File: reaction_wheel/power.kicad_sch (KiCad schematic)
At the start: 20 parts, among them U10 TPS62902RPJR, U11 TPS61379QWRTERQ1

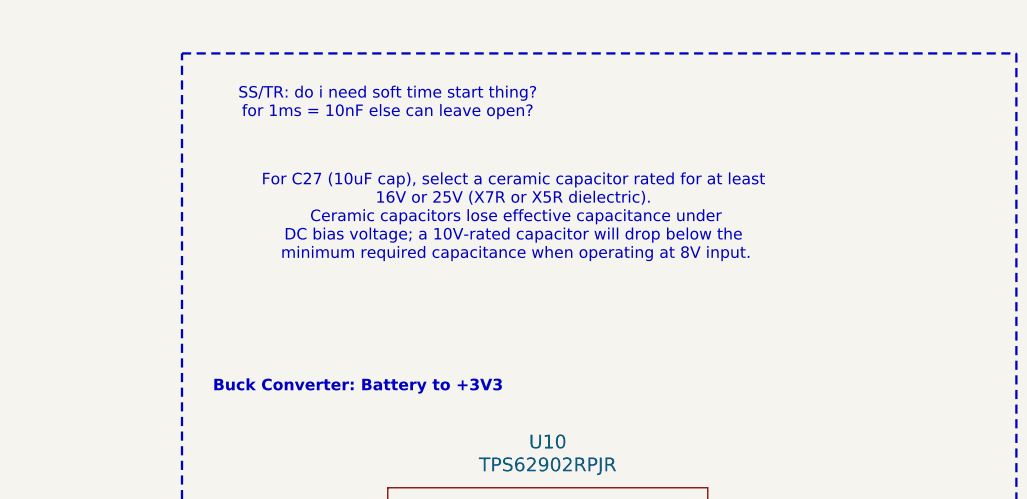
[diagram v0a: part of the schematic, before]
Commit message: added notes
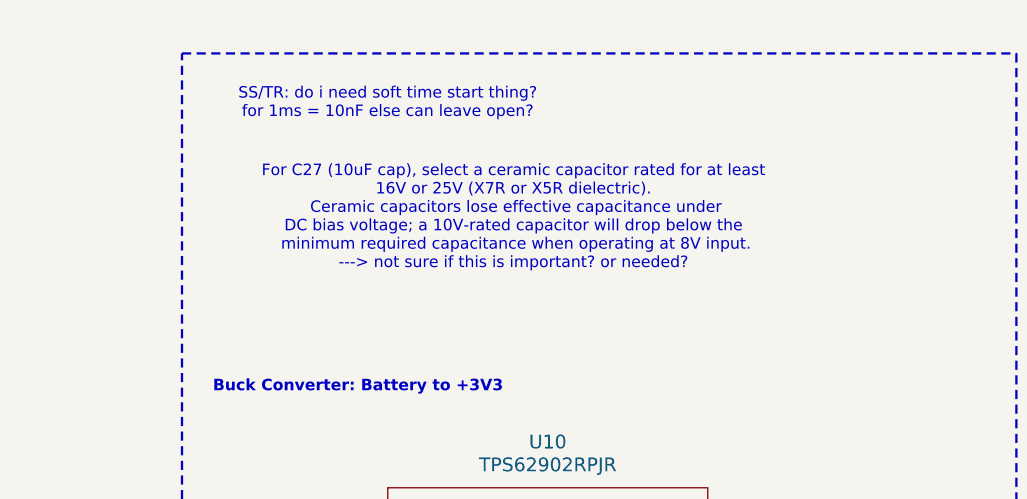
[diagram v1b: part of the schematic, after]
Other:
- note added: "For C27 (10uF cap), select a ceramic capacitor rated for at least 16V or 25V (X7R or X5R dielectric). Ceramic capacitors lose effective capacitance under DC bias voltage; a 10V-rated capacitor will drop below the minimum required capacitance when operating at 8V input. ---> not sure if this is important? or needed?"
- note removed: "For C27 (10uF cap), select a ceramic capacitor rated for at least 16V or 25V (X7R or X5R dielectric). Ceramic capacitors lose effective capacitance under DC bias voltage; a 10V-rated capacitor will drop below the minimum required capacitance when operating at 8V input."
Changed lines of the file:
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@@
 		)
 	)
-	(text "For C27 (10uF cap), select a ceramic capacitor rated for at least \n16V or 25V (X7R or X5R dielectric).\n Ceramic capacitors lose effective capacitance under \nDC bias voltage; a 10V-rated capacitor will drop below the\n minimum required capacitance when operating at 8V input."
+	(text "For C27 (10uF cap), select a ceramic capacitor rated for at least \n16V or 25V (X7R or X5R dielectric).\n Ceramic capacitors lose effective capacitance under \nDC bias voltage; a 10V-rated capacitor will drop below the\n minimum required capacitance when operating at 8V input.\n---> not sure if this is important? or needed? "
 		(exclude_from_sim no)
 		(at 199.39 38.608 0)
